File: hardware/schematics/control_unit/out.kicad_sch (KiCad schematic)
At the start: 50 parts, among them Q1 IRFZ44N, Q10 IRFZ44N, Q2 IRFZ44N, Q3 IRFZ44N, Q4 IRFZ44N, Q5 IRFZ44N, Q6 IRFZ44N, Q7 IRFZ44N, Q8 IRFZ44N, Q9 IRFZ44N, U1 PC817, U10 PC817, U2 PC817, U3 PC817, U4 PC817, U5 PC817, U6 PC817, U7 PC817, U8 PC817, U9 PC817

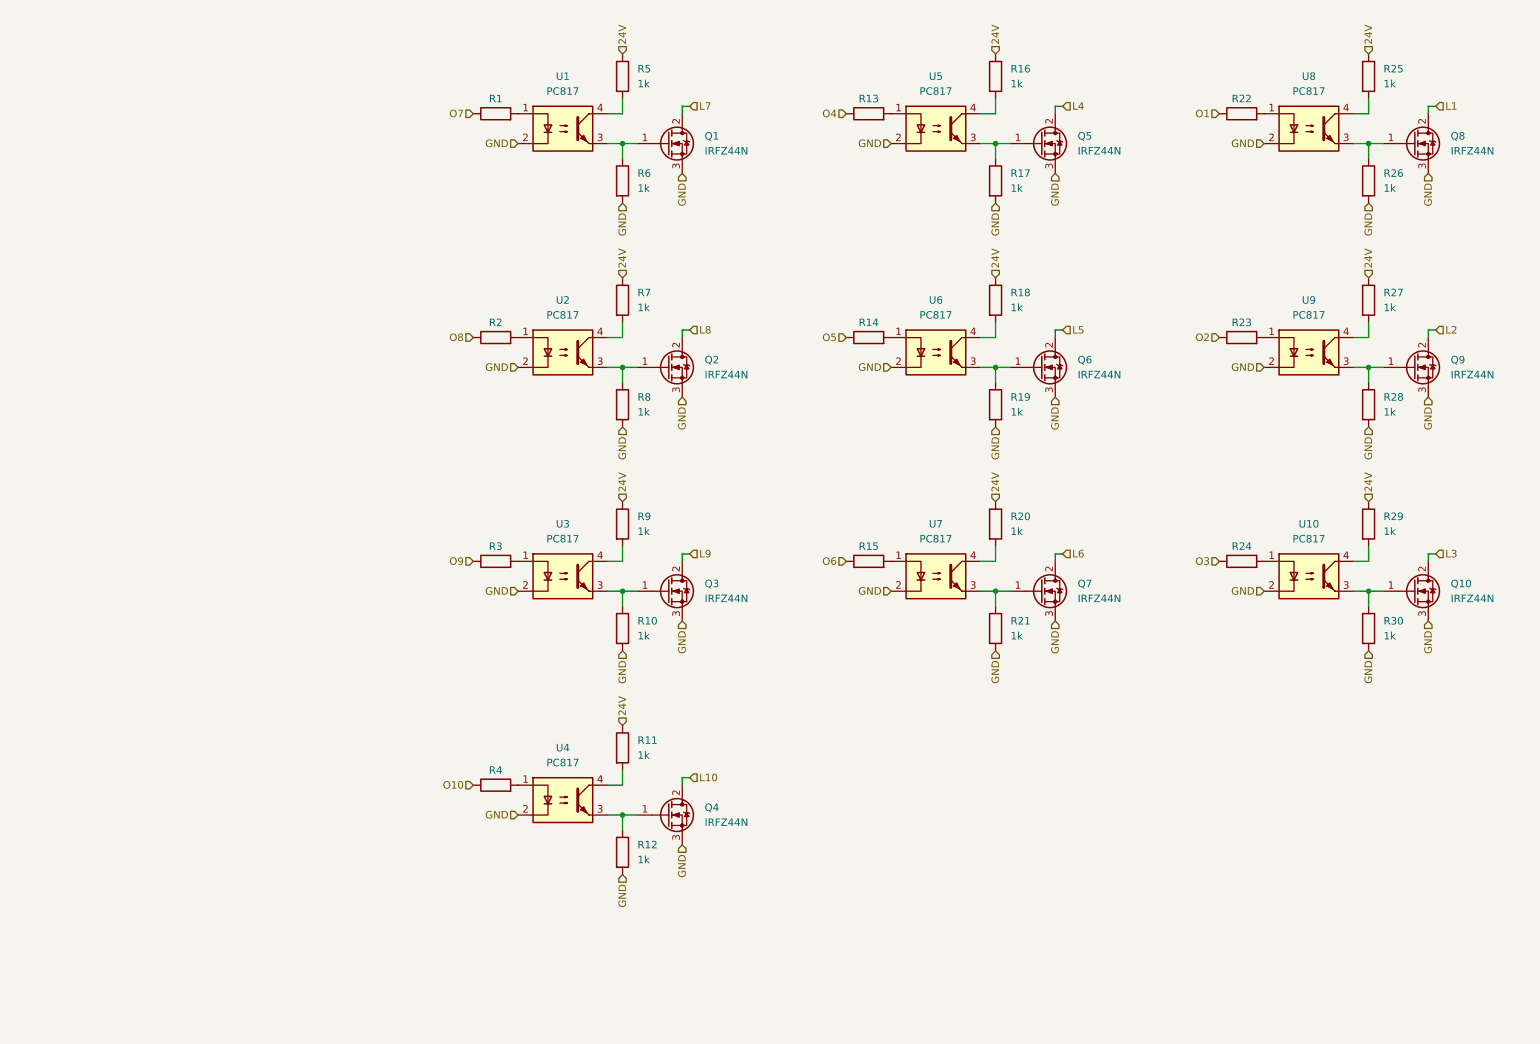
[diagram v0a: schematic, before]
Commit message: feat
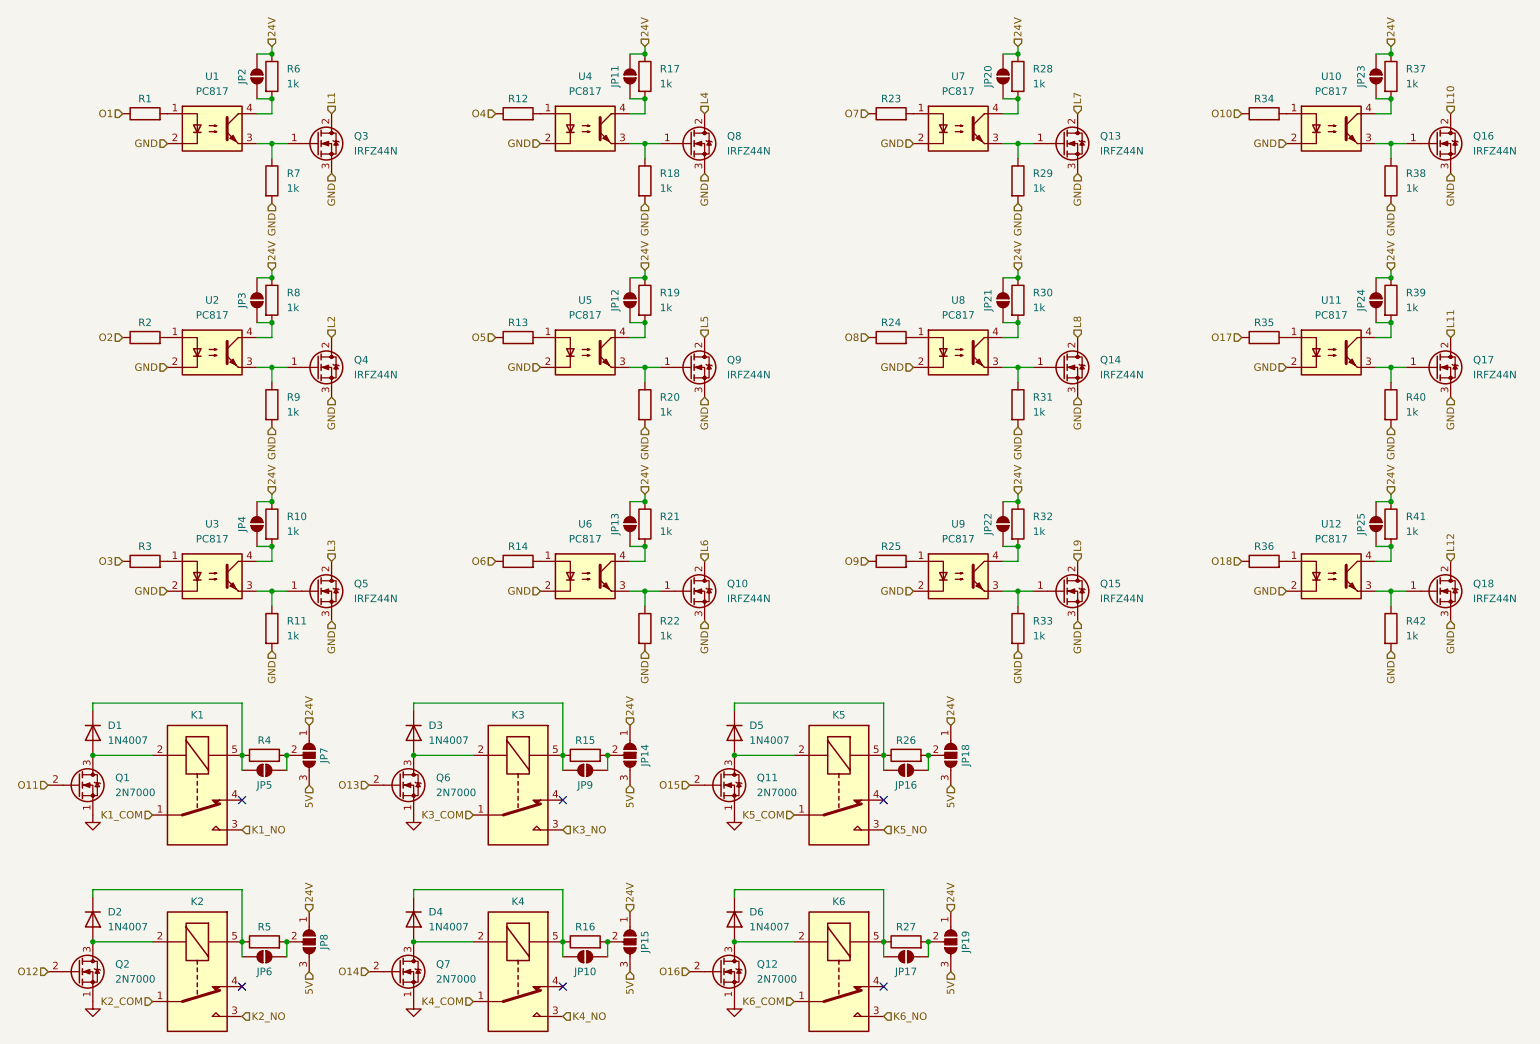
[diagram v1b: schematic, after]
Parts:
- removed Q10, Q4, Q8, Q9: IRFZ44N, Package_TO_SOT_THT:TO-220-3_Vertical, symbol Transistor_FET:IRF540N
- removed R11, R12: 1k, symbol Device:R
- removed R22: R, symbol Device:R
- removed U4: PC817, Package_DIP:DIP-4_W7.62mm, symbol Isolator:PC817
- added D1, D2, D3, D4, D5, D6: 1N4007, Diode_THT:D_DO-41_SOD81_P2.54mm_Vertical_KathodeUp, symbol Diode:1N4007
- added JP10, JP11, JP12, JP13, JP16, JP17, JP2, JP20, JP21, JP22, JP23, JP24, JP25, JP3, JP4, JP5, JP6, JP9: SolderJumper_2_Open, symbol Jumper:SolderJumper_2_Open
- added JP14, JP15, JP18, JP19, JP7, JP8: SolderJumper_3_Open, Jumper:SolderJumper-3_P1.3mm_Open_Pad1.0x1.5mm, symbol Jumper:SolderJumper_3_Open
- added K1, K2, K3, K4, K5, K6: Relay_SPDT, Relay_THT:Relay_SPDT_Omron-G5LE-1, symbol Relay:Relay_SPDT
- added Q1, Q11, Q12, Q2, Q6, Q7: 2N7000, Package_TO_SOT_THT:TO-92_Inline, symbol Transistor_FET:2N7000
- added Q13, Q14, Q15, Q16, Q17, Q18: IRFZ44N, Package_TO_SOT_THT:TO-220-3_Vertical, symbol Transistor_FET:IRF540N
- added R15, R16, R34, R35, R36, R5: R, symbol Device:R
- added R31, R32, R33, R37, R38, R39, R40, R41, R42: 1k, symbol Device:R
- added U11, U12, U7: PC817, Package_DIP:DIP-4_W7.62mm, symbol Isolator:PC817
- R25, R26, R27: value 1k -> R
- renumbered Q7 to Q10, Q1 to Q3, Q2 to Q4, Q3 to Q5, Q5 to Q8, Q6 to Q9, R9 to R10, R10 to R11, R13 to R12, R14 to R13, R15 to R14, R16 to R17, R17 to R18, R18 to R19, R19 to R20, R20 to R21, R21 to R22, R5 to R6, R6 to R7, R7 to R8, R8 to R9, U5 to U4, U6 to U5, U7 to U6
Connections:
- net 24V: now also R28.1, R30.1, JP11.2 (B), JP12.2 (B), JP13.2 (B), JP14.1 (A), JP15.1 (A), JP18.1 (A), JP19.1 (A), JP2.2 (B), JP20.2 (B), JP21.2 (B), JP22.2 (B), JP23.2 (B), JP24.2 (B), JP25.2 (B), JP3.2 (B), JP4.2 (B), JP7.1 (A), JP8.1 (A), R32.1, R37.1, R39.1, R41.1; no longer R25.1, R27.1, R29.1
- net GND: now also R29.2, Q1.1 (S), Q11.1 (S), Q12.1 (S), Q13.3 (S), Q14.3 (S), Q15.3 (S), Q16.3 (S), Q17.3 (S), Q18.3 (S), Q2.1 (S), Q6.1 (S), Q7.1 (S), R31.2, R33.2, R38.2, R40.2, R42.2, U11.2, U12.2, U7.2; no longer R26.2, R28.2, R30.2
- net L1: now also Q3.2 (D)
- net L10: now also Q16.2 (D)
- net L2: now also Q4.2 (D)
- net L3: now also Q5.2 (D)
- net L7: now also Q13.2 (D); no longer Q3.2 (D)
- net L8: now also Q14.2 (D); no longer Q4.2 (D)
- net L9: now also Q15.2 (D); no longer Q5.2 (D)
- net O1: now also R1.1
- net O10: now also R34.1; no longer R4.1
- net O2: now also R2.1; no longer R23.1
- net O3: now also R3.1; no longer R24.1
- net O7: now also R23.1; no longer R1.1
- net O8: now also R24.1; no longer R2.1
- net O9: now also R25.1; no longer R3.1
- net at R8.2, U2.4: now also JP3.1 (A)
- net at R10.2, U3.4: now also JP4.1 (A)
- net at R4.2: now also JP5.1 (A), JP7.2 (C)
- net at U10.1: now also R34.2; no longer R24.2
- net at U10.3: now also Q16.1 (G), R38.1; no longer R30.1
- net at U10.4: now also JP23.1 (A), R37.2; no longer R29.2
- net at U9.3: now also Q15.1 (G), R33.1; no longer R28.1
- net at R17.2, U4.4: now also JP11.1 (A)
- net at R21.2, U6.4: now also JP13.1 (A)
- net at R26.1: now also D5.1 (K), JP16.2 (B), K5.5; no longer U8.3
- net at R19.2, U5.4: now also JP12.1 (A)
- net at U8.1: now also R24.2
- net at R6.2, U1.4: now also JP2.1 (A)
- net at R25.2: now also U9.1; no longer U8.4
- net at R23.2: now also U7.1; no longer U9.1
- net at R27.2: now also JP17.1 (A), JP19.2 (C); no longer U9.4
- new net: D3.2 (A), K3.2, Q6.3 (D)
- new net: D3.1 (K), JP9.2 (B), K3.5, R15.1
- new net: JP14.2 (C), JP9.1 (A), R15.2
- new net: Q17.1 (G), R40.1, U11.3
- new net: D6.2 (A), K6.2, Q12.3 (D)
- new net: D1.1 (K), JP5.2 (B), K1.5, R4.1
- new net: D1.2 (A), K1.2, Q1.3 (D)
- new net: JP16.1 (A), JP18.2 (C), R26.2
- new net: D2.2 (A), K2.2, Q2.3 (D)
- new net: D2.1 (K), JP6.2 (B), K2.5, R5.1
- new net: JP22.1 (A), R32.2, U9.4
- new net: JP6.1 (A), JP8.2 (C), R5.2
- new net: R35.2, U11.1
- new net: JP24.1 (A), R39.2, U11.4
- new net: D4.1 (K), JP10.2 (B), K4.5, R16.1
- new net: JP10.1 (A), JP15.2 (C), R16.2
- new net: D4.2 (A), K4.2, Q7.3 (D)
- new net: D6.1 (K), JP17.2 (B), K6.5, R27.1
- new net: JP20.1 (A), R28.2, U7.4
- new net: Q13.1 (G), R29.1, U7.3
- new net: JP25.1 (A), R41.2, U12.4
- new net: JP21.1 (A), R30.2, U8.4
- new net: D5.2 (A), K5.2, Q11.3 (D)
- new net: Q14.1 (G), R31.1, U8.3
- new net: Q18.1 (G), R42.1, U12.3
- new net: R36.2, U12.1
- new net 5V: JP14.3 (B), JP15.3 (B), JP18.3 (B), JP19.3 (B), JP7.3 (B), JP8.3 (B)
- new net K1_COM: K1.1
- new net K1_NO: K1.3
- new net K2_COM: K2.1
- new net K2_NO: K2.3
- new net K3_COM: K3.1
- new net K3_NO: K3.3
- new net K4_COM: K4.1
- new net K4_NO: K4.3
- new net K5_COM: K5.1
- new net K5_NO: K5.3
- new net K6_COM: K6.1
- new net K6_NO: K6.3
- new net L11: Q17.2 (D)
- new net L12: Q18.2 (D)
- new net O11: Q1.2 (G)
- new net O12: Q2.2 (G)
- new net O13: Q6.2 (G)
- new net O14: Q7.2 (G)
- new net O15: Q11.2 (G)
- new net O16: Q12.2 (G)
- new net O17: R35.1
- new net O18: R36.1
- no-connect marks 0 -> 6
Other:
- moved on the sheet: Q10, Q3, Q4, Q5, Q8, Q9, R1, R10, R11, R12, R13, R14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
